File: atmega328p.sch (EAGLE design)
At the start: 6 parts, among them IC1 ATMEGA328-20P, X1 CRYSTALS-NOGND-HC49

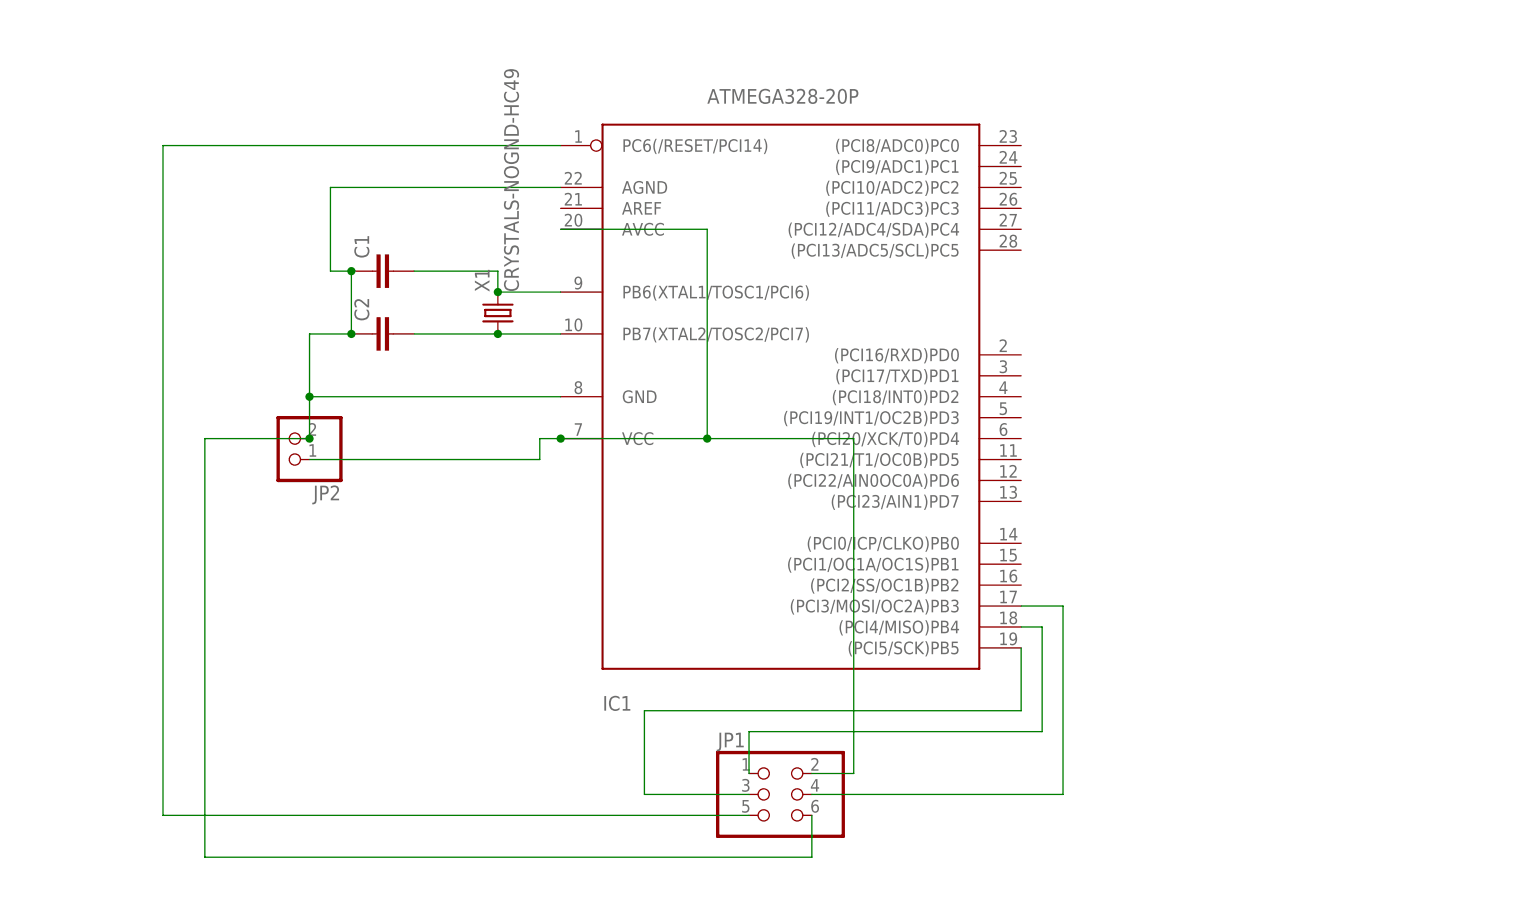
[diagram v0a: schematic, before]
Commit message: with PCB bord
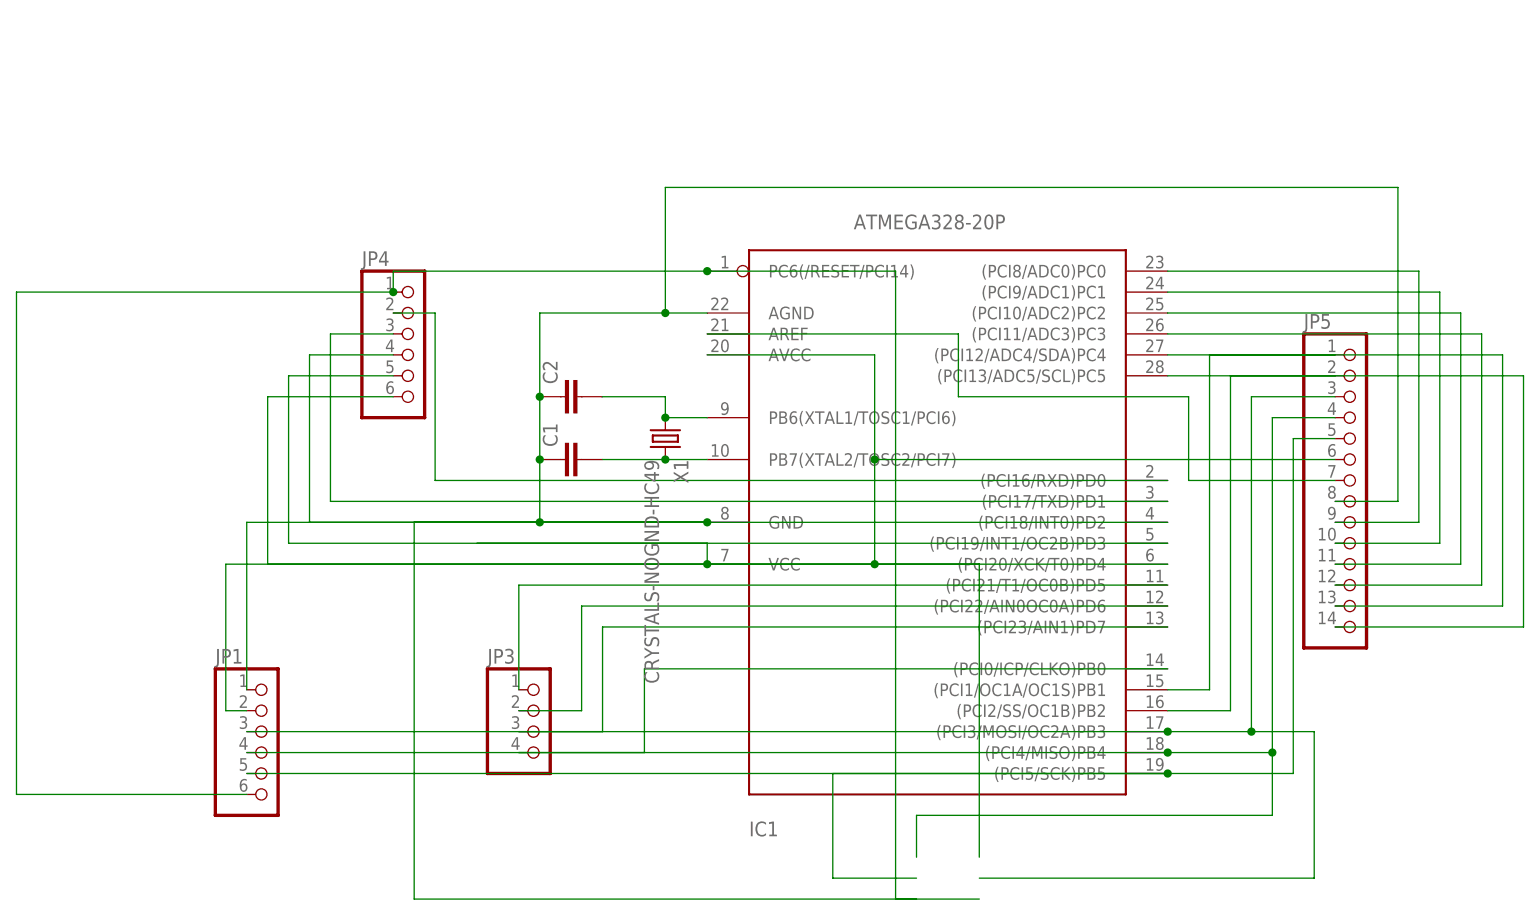
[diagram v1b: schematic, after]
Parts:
- removed JP2: (no value), pinhead:PINHD-1X2
- added JP3: (no value), pinhead:PINHD-1X4
- added JP4: (no value), pinhead:PINHD-1X6
- added JP5: (no value), pinhead:PINHD-1X14
- JP1: device pinhead:PINHD-2X3 -> pinhead:PINHD-1X6
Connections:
- new net N$11: IC1.(PCI18/INT0)PD2, JP4.4
- new net N$12: IC1.(PCI19/INT1/OC2B)PD3, JP4.5
- new net N$13: IC1.(PCI20/XCK/T0)PD4, JP4.6
- new net N$14: IC1.(PCI21/T1/OC0B)PD5, JP3.1
- new net N$15: IC1.(PCI22/AIN0OC0A)PD6, JP3.2
- new net N$16: IC1.(PCI23/AIN1)PD7, JP3.3
- new net N$17: IC1.(PCI0/ICP/CLKO)PB0, JP3.4
- new net N$18: IC1.(PCI1/OC1A/OC1S)PB1, JP5.1
- new net N$19: IC1.(PCI2/SS/OC1B)PB2, JP5.2
- new net N$21: IC1.(PCI8/ADC0)PC0, JP5.9
- new net N$22: IC1.(PCI9/ADC1)PC1, JP5.10
- new net N$23: IC1.AREF, JP5.7
- new net N$24: IC1.(PCI10/ADC2)PC2, JP5.11
- new net N$25: IC1.(PCI11/ADC3)PC3, JP5.12
- new net N$26: IC1.(PCI12/ADC4/SDA)PC4, JP5.13
- new net N$27: IC1.(PCI13/ADC5/SCL)PC5, JP5.14
- new net N$5: C1.1, C2.1, IC1.AGND, IC1.GND, JP1.1, JP5.8
- new net N$6: IC1.(PCI17/TXD)PD1, JP4.3
- net N$1: now also IC1.AVCC, IC1.VCC, JP1.2, JP5.6; no longer C1.2, IC1.PB6(XTAL1/TOSC1/PCI6), X1.2
- net N$10: now also IC1.(PCI5/SCK)PB5, JP1.5, JP5.5; no longer IC1.(PCI3/MOSI/OC2A)PB3, JP1.4
- net N$2: now also IC1.(PCI16/RXD)PD0, JP4.2; no longer C2.2, IC1.PB7(XTAL2/TOSC2/PCI7), X1.1
- net N$3: now also C2.2, IC1.PB6(XTAL1/TOSC1/PCI6), X1.1; no longer C1.1, C2.1, IC1.AGND, IC1.GND, JP1.6, JP2.2
- net N$4: now also C1.2, IC1.PB7(XTAL2/TOSC2/PCI7), X1.2; no longer IC1.AVCC, IC1.VCC, JP1.2, JP2.1
- net N$7: now also JP1.6, JP4.1; no longer JP1.5
- net N$8: now also IC1.(PCI3/MOSI/OC2A)PB3, JP5.3; no longer IC1.(PCI5/SCK)PB5
- net N$9: now also JP1.4, JP5.4; no longer JP1.1
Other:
- moved on the sheet: C1, C2, IC1, JP1, X1
